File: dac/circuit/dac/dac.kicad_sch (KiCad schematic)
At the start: 10 parts, among them J1 DB25_Socket, U1 MCP4922-EP, U2 MCP4922-EP, U3 L7805, U4 TL074BCDT, U5 ADUM1401BRWZ, U6 ADUM1401BRWZ, U7 MCP4922-EP

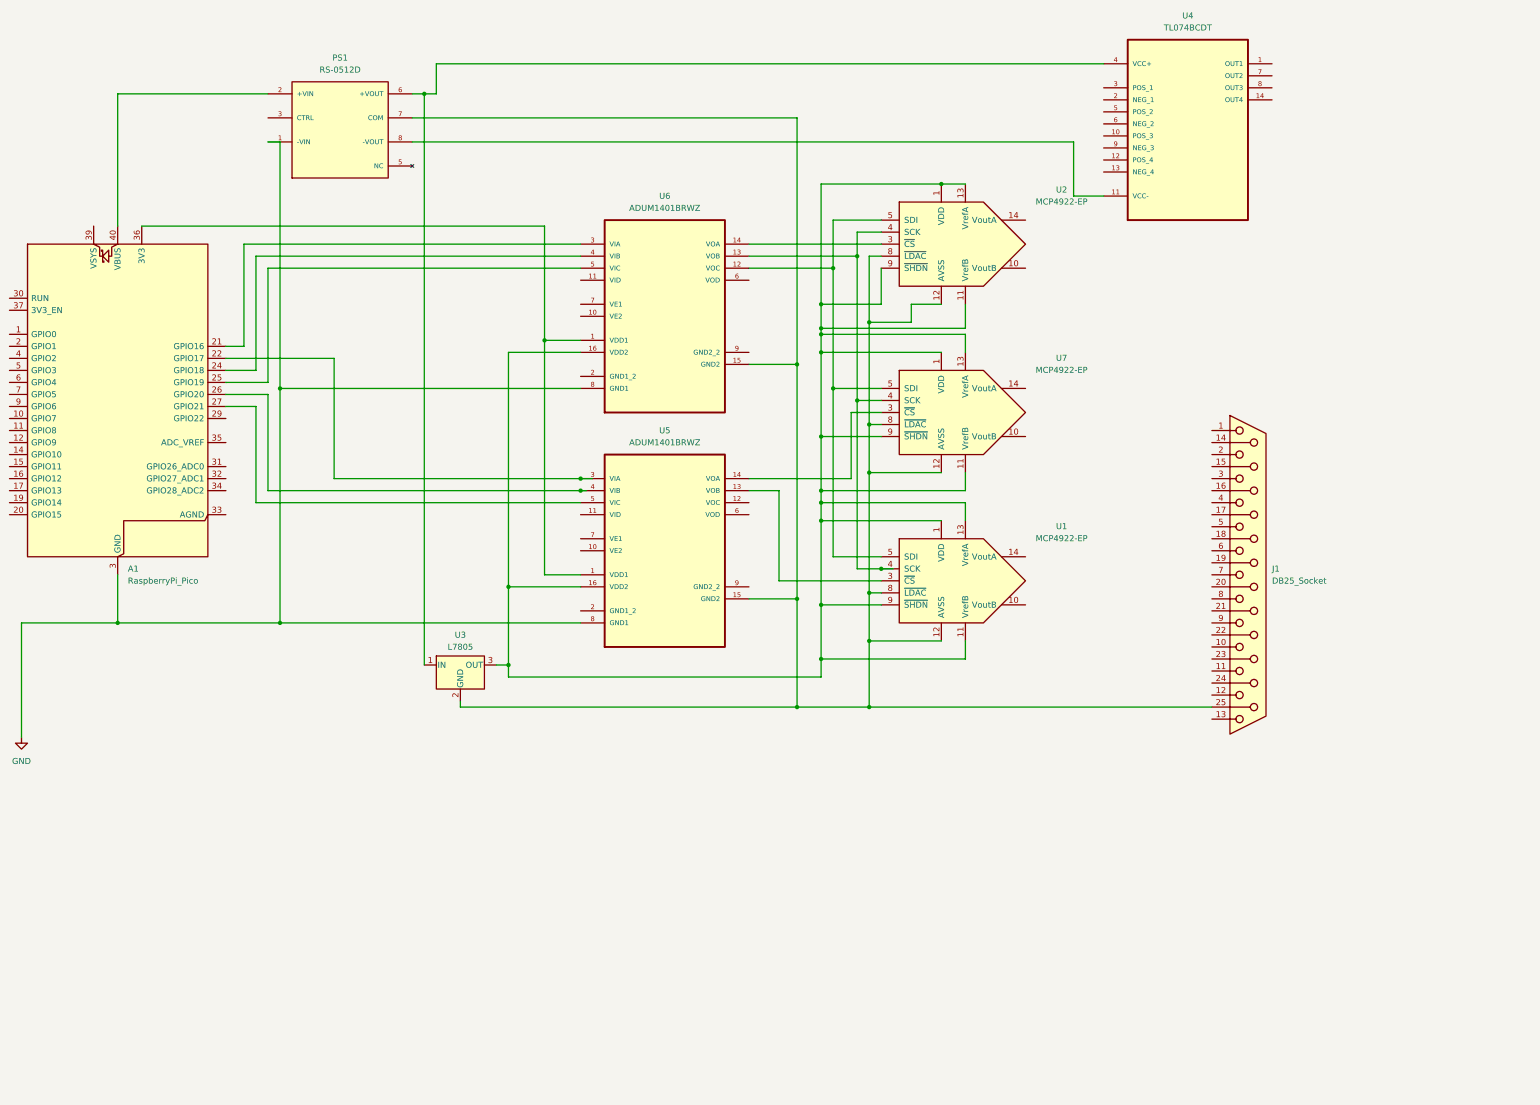
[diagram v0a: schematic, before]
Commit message: add testst
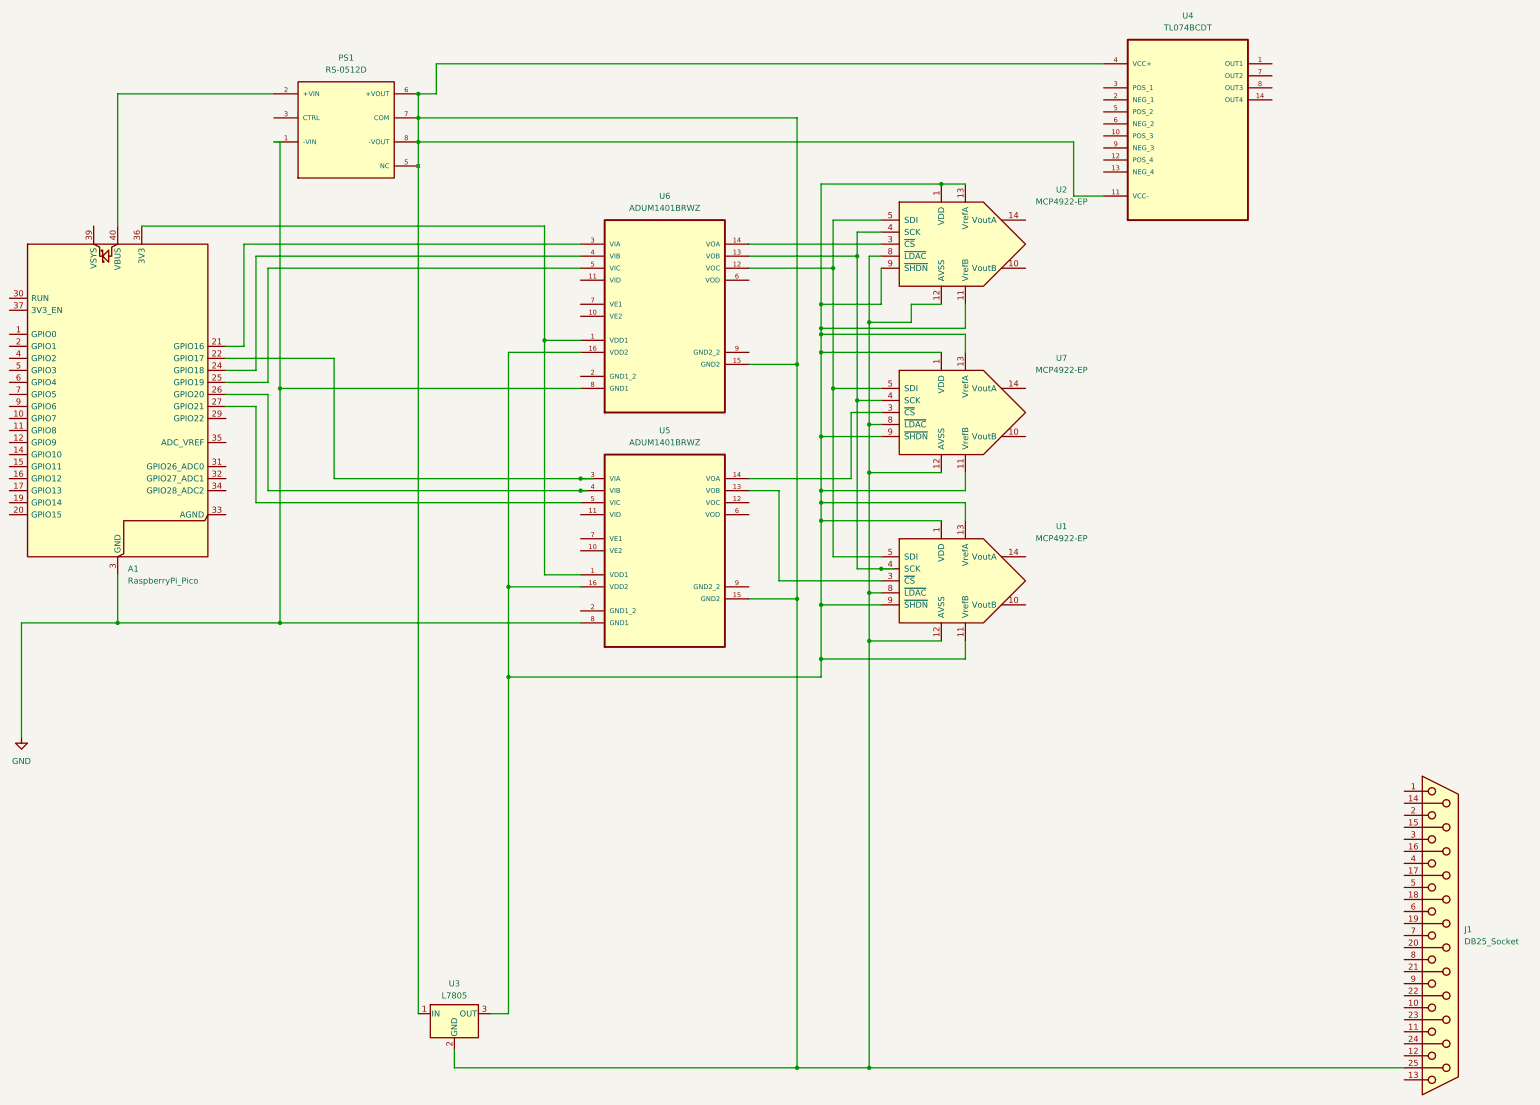
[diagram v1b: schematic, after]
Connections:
- net at PS1.6 (+VOUT), U3.1 (IN), U4.4 (VCC+): now also J1.25 (P25), PS1.7 (COM), PS1.8 (-VOUT), U1.12 (AVSS), U1.8 (~{LDAC}), U2.12 (AVSS), U2.8 (~{LDAC}), U3.2 (GND), U4.11 (VCC-), U5.15 (GND2), U6.15 (GND2), U7.12 (AVSS), U7.8 (~{LDAC})
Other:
- moved on the sheet: J1, PS1, U3
